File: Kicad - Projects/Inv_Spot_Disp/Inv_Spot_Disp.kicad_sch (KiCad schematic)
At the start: 38 parts, among them J1 PWM_Out, J2 Power_Supply, J3 Trigger, J4 Prog, SW1 1, SW2 2, SW3 3, SW4 4, SW5 SW_Push, U1 STM32F030F4Px, U2 NHD-0420H1Z, U3 AMS1117-3.3, U4 LKS561, U5 L7805, U6 LTV-817S

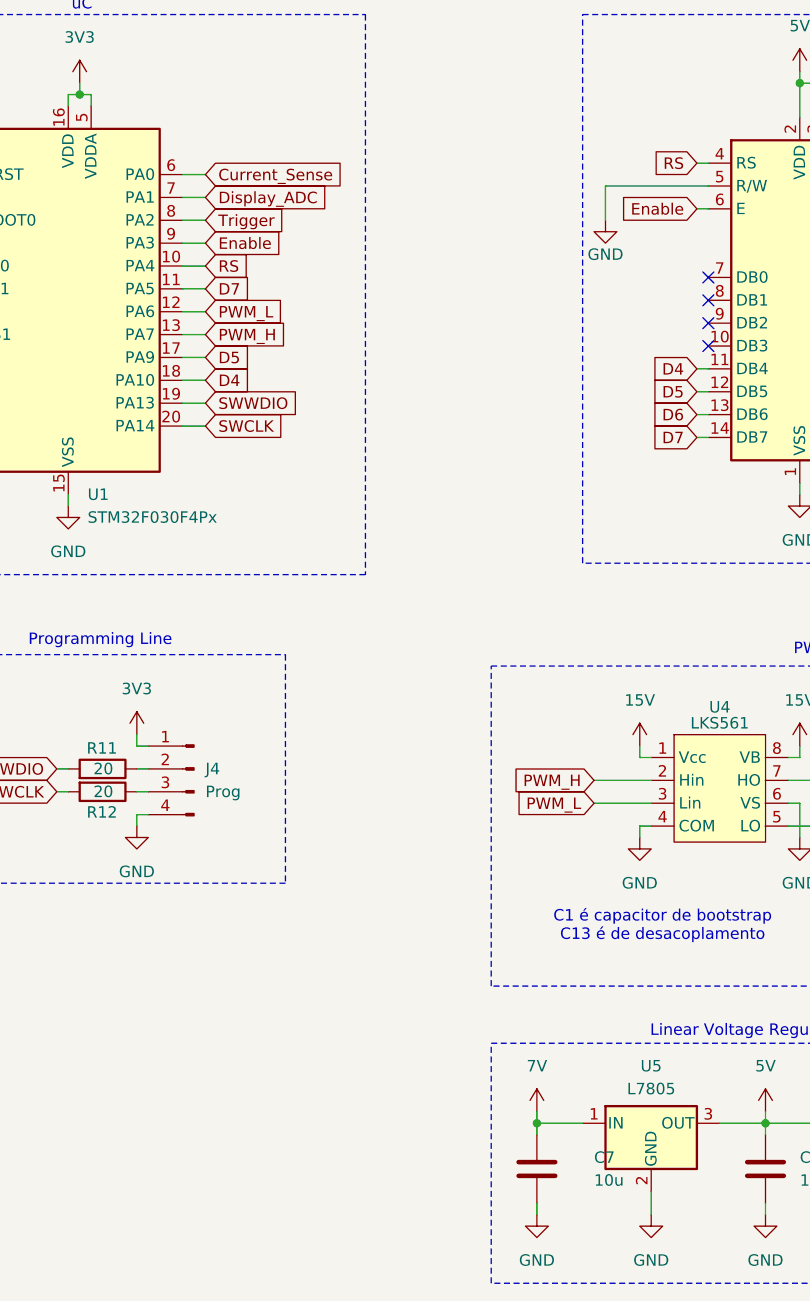
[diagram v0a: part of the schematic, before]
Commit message: Cotações
Cotações
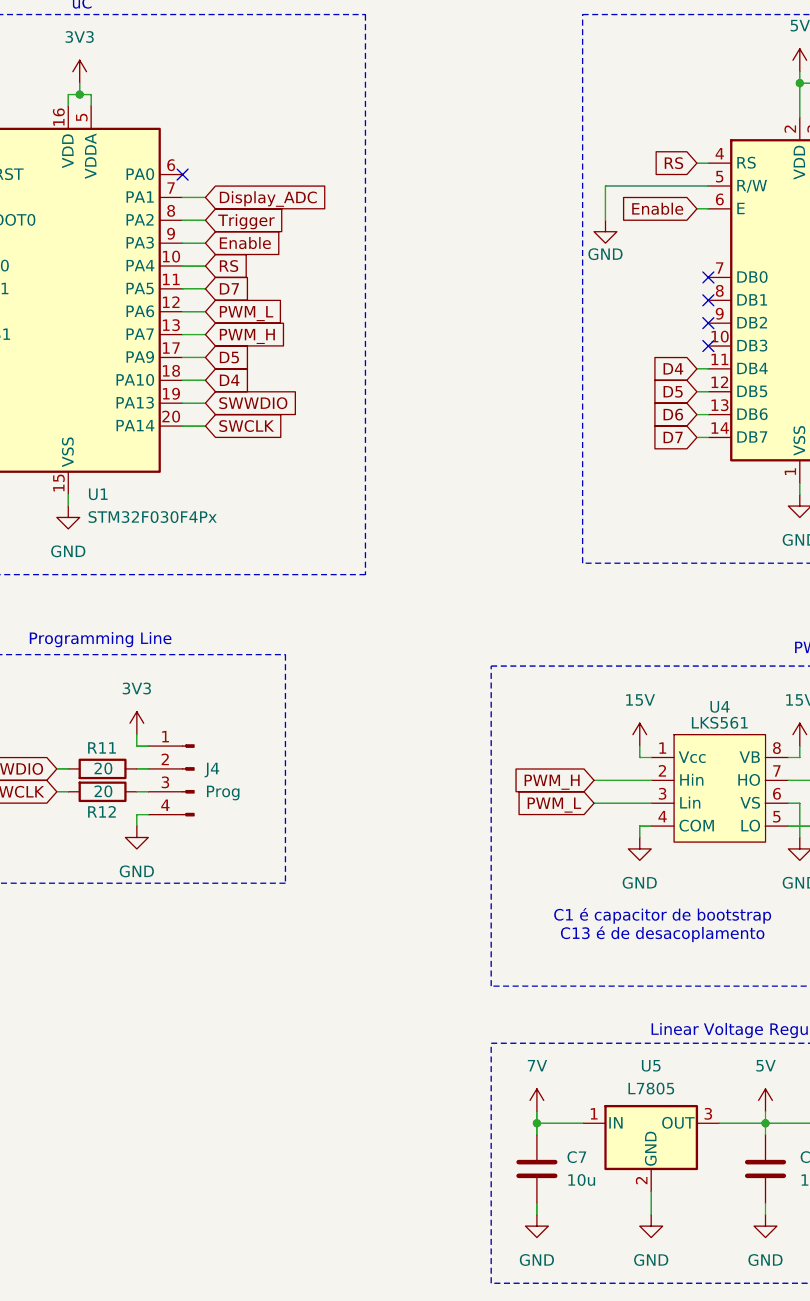
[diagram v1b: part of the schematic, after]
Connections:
- net Current_Sense: no longer names the net of U1.6 (PA0)
- no-connect marks 7 -> 8
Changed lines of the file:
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@@
+	)
+	(no_connect
+		(at 143.51 38.1)
 	)
 	(no_connect
@@
 		(pts
 			(xy 130.81 30.48) (xy 130.81 29.21)
-		)
-		(stroke
-			(width 0)
-			(type default)
-		)
-	)
-	(wire
-		(pts
-			(xy 143.51 38.1) (xy 146.05 38.1)
 		)
 		(stroke
@@
 		(property "Intersheetrefs" "${INTERSHEET_REFS}"
 			(at 151.5147 50.8 0)
-			(hide yes)
-			(show_name no)
-			(do_not_autoplace no)
-			(effects
-				(font
-					(size 1.27 1.27)
-				)
-				(justify left)
-			)
-		)
-	)
-	(global_label "Current_Sense"
-		(shape input)
-		(at 146.05 38.1 0)
-		(fields_autoplaced yes)
-		(effects
-			(font
-				(size 1.27 1.27)
-			)
-			(justify left)
-		)
-		(property "Intersheetrefs" "${INTERSHEET_REFS}"
-			(at 162.5213 38.1 0)
 			(hide yes)
 			(show_name no)
@@
 		(dnp no)
 		(property "Reference" "C7"
-			(at 189.23 147.3199 0)
+			(at 186.182 147.32 0)
 			(show_name no)
 			(do_not_autoplace no)
@@
 		)
 		(property "Value" "10u"
-			(at 189.23 149.8599 0)
-			(show_name no)
-			(do_not_autoplace no)
+			(at 186.182 149.86 0)
+			(show_name no)
+			(do_not_autoplace no)
